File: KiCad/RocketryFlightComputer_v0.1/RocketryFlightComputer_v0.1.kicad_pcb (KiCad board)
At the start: 4 copper layers, 25.4 x 31.8 mm, 34 parts, among them J1 USB_C_Receptacle, J2 Conn_Coaxial, J3 DEPLOYMENT, J4 POWER_IN, Q1 BSS806NH6327XTSA1, Q2 BSS806NH6327XTSA1, Q3 BSS806NH6327XTSA1, U1 STM32U545RET6Q, U2 SX1262IMLTRT, U3 W25N01GWZEIG, U4 BME680, U5 MMC5633NJL, U6 TLV77118PDBVR, U7 ICM-20602, U8 TPS63070RNMR, U9 EVA-M8M-0, Y1 END4263D-32M, Y2 SIT1552AI-JE-DCC-32.768E

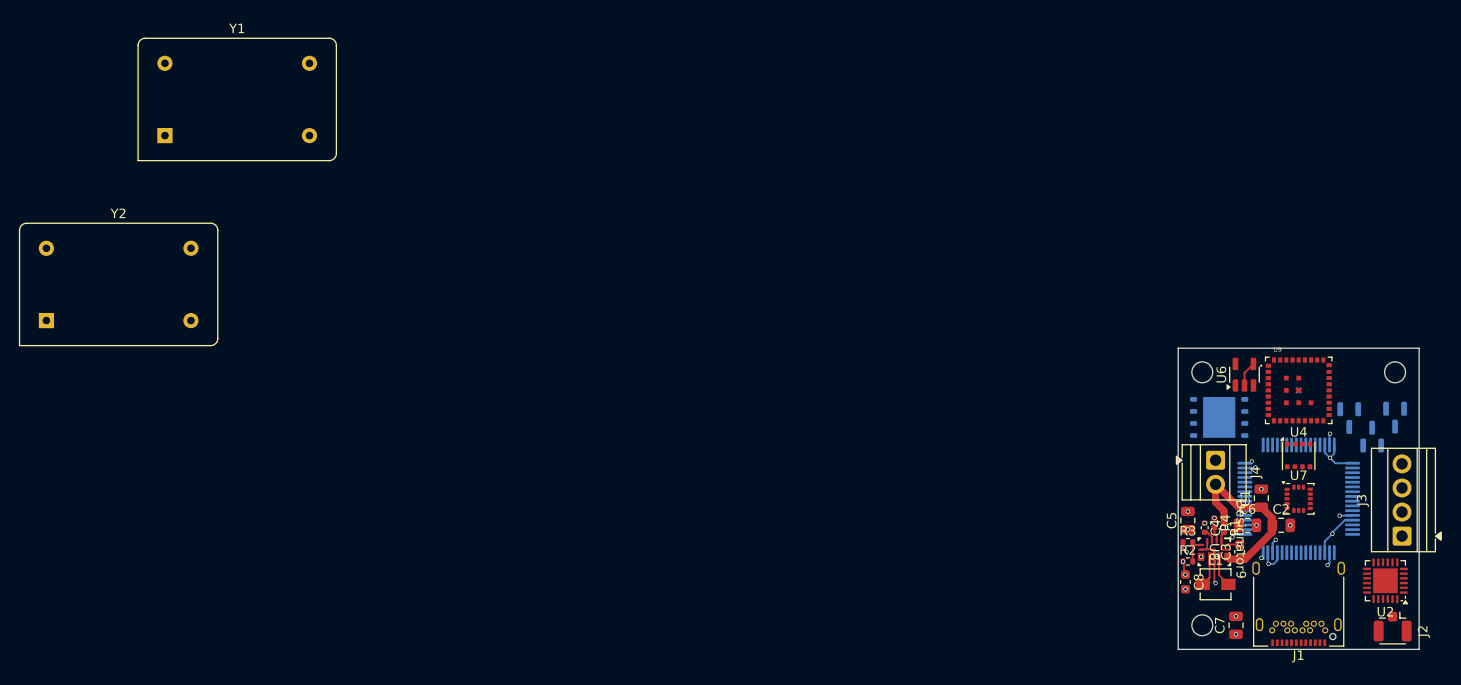
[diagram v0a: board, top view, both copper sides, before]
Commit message: Finished Board v0.1
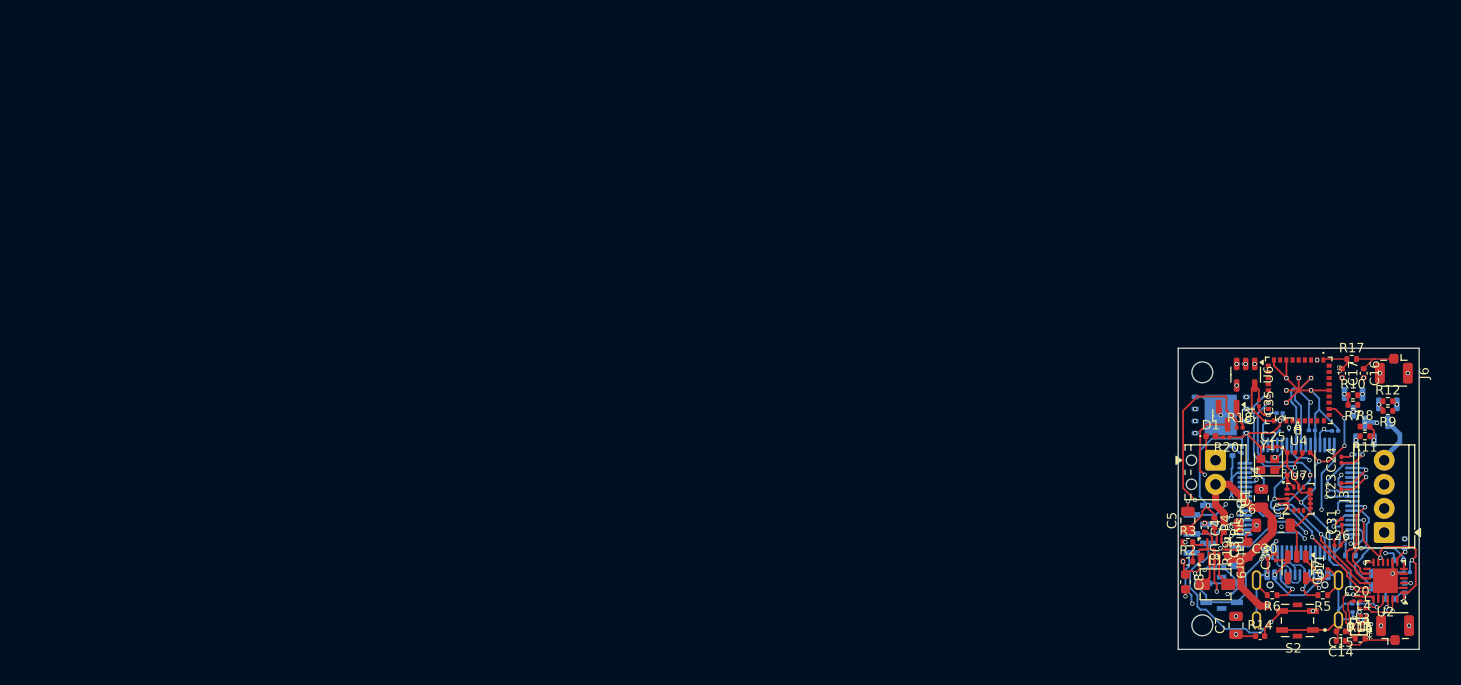
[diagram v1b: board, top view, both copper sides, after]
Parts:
- removed the REF** at (226.1, 88.3)
- added C10: 2.2u, Resistor_SMD:R_0402_1005Metric, B.Cu at (208.9, 96.5)
- added C11: 10p, Resistor_SMD:R_0402_1005Metric, B.Cu at (227.1, 111.0)
- added C12: 100n, Resistor_SMD:R_0402_1005Metric, B.Cu at (226.4, 108.1)
- added C13: 470u, Capacitor_SMD:C_0402_1005Metric, B.Cu at (227.1, 106.3)
- added C14: 0, Capacitor_SMD:C_0402_1005Metric, F.Cu at (220.3, 116.6)
- added C15: 0, Capacitor_SMD:C_0402_1005Metric, F.Cu at (220.3, 115.6)
- added C16: 0, Capacitor_SMD:C_0402_1005Metric, F.Cu at (222.8, 88.4)
- added C17: 0, Capacitor_SMD:C_0402_1005Metric, F.Cu at (220.5, 88.4)
- added C18: 1.5p, Capacitor_SMD:C_0201_0603Metric, B.Cu at (221.9, 113.5)
- added C19: 1p, Capacitor_SMD:C_0201_0603Metric, B.Cu at (222.4, 114.3)
- added C20: 1p, Capacitor_SMD:C_0201_0603Metric, F.Cu at (222.0, 112.4)
- added C21: 100p, Capacitor_SMD:C_0201_0603Metric, B.Cu at (224.4, 114.6)
- added C22: 100n, Capacitor_SMD:C_0201_0603Metric, B.Cu at (219.7, 94.4)
- added C23: 10u, Capacitor_SMD:C_0201_0603Metric, F.Cu at (220.4, 100.3)
- added C24: 10u, Capacitor_SMD:C_0201_0603Metric, F.Cu at (220.4, 97.5)
- added C25: 4.7u, Capacitor_SMD:C_0201_0603Metric, F.Cu at (213.2, 96.1)
- added C26: 1u, Capacitor_SMD:C_0201_0603Metric, F.Cu at (220.0, 106.5)
- added C27: 100n, Capacitor_SMD:C_0201_0603Metric, B.Cu at (222.1, 96.9)
- added C28: 100n, Capacitor_SMD:C_0201_0603Metric, B.Cu at (217.3, 94.4)
- added C29: 100n, Capacitor_SMD:C_0201_0603Metric, B.Cu at (209.9, 96.4)
- added C30: 100n, Capacitor_SMD:C_0201_0603Metric, F.Cu at (212.3, 107.9)
- added C31: 1u, Capacitor_SMD:C_0201_0603Metric, F.Cu at (220.4, 104.0)
- added C32: 2.2u, Capacitor_SMD:C_0201_0603Metric, B.Cu at (227.3, 109.3)
- added C33: 10u, Capacitor_SMD:C_0201_0603Metric, B.Cu at (213.9, 92.6)
- added C34: 10u, Capacitor_SMD:C_0201_0603Metric, B.Cu at (209.8, 87.4)
- added C35: 10u, Capacitor_SMD:C_0201_0603Metric, F.Cu at (211.7, 91.5)
- added C36: 2.2u, Capacitor_SMD:C_0201_0603Metric, F.Cu at (213.5, 107.8)
- added C37: 2.2u, Capacitor_SMD:C_0201_0603Metric, F.Cu at (218.9, 109.3)
- added C9: 2.2u, Resistor_SMD:R_0402_1005Metric, B.Cu at (221.4, 107.6)
- added D1: LED, LED_SMD:LED_0402_1005Metric, F.Cu at (206.6, 95.0)
- added J5: USB_C_Receptacle_USB2.0_16P, Connector_USB:USB_C_Receptacle_GCT_USB4105-xx-A_16P_TopMnt_Horizontal, B.Cu at (215.8, 113.3)
- added J6: Conn_Coaxial, Connector_Coaxial:U.FL_Hirose_U.FL-R-SMT-1_Vertical, F.Cu at (225.9, 87.9)
- added L2: 2.2u, Capacitor_SMD:C_0805_2012Metric, B.Cu at (209.4, 107.6)
- added L3: 3.9n, Inductor_SMD:L_0201_0603Metric, F.Cu at (222.6, 113.2)
- added L4: 6.8n, Inductor_SMD:L_0201_0603Metric, F.Cu at (222.8, 113.9)
- added L5: 8.2n, Inductor_SMD:L_0201_0603Metric, B.Cu at (221.9, 112.6)
- added Q4: BSS806NH6327XTSA1, Package_TO_SOT_SMD:SOT-23, F.Cu at (208.4, 92.8)
- added R10: 10k, Resistor_SMD:R_0402_1005Metric, F.Cu at (221.6, 90.7)
- added R11: 10k, Resistor_SMD:R_0402_1005Metric, F.Cu at (222.9, 95.0)
- added R12: 10k, Resistor_SMD:R_0402_1005Metric, F.Cu at (225.3, 91.3)
- added R13: 220, Resistor_SMD:R_0402_1005Metric, B.Cu at (225.6, 112.1)
- added R14: 10k, Capacitor_SMD:C_0402_1005Metric, F.Cu at (211.8, 116.1)
- added R15: 10k, Capacitor_SMD:C_0402_1005Metric, B.Cu at (207.5, 108.8)
- added R16: 0, Resistor_SMD:R_0402_1005Metric, F.Cu at (222.4, 116.3)
- added R17: 0, Resistor_SMD:R_0402_1005Metric, F.Cu at (221.5, 86.9)
- added R18: 10k, Resistor_SMD:R_0201_0603Metric, F.Cu at (209.7, 94.1)
- added R19: 100k, Resistor_SMD:R_0201_0603Metric, F.Cu at (209.4, 107.3)
- added R20: 330, Resistor_SMD:R_0201_0603Metric, F.Cu at (208.3, 95.1)
- added R5: 5.1k, Resistor_SMD:R_0402_1005Metric, F.Cu at (218.4, 111.8)
- added R6: 5.1k, Resistor_SMD:R_0402_1005Metric, F.Cu at (213.1, 111.8)
- added R7: 100, Resistor_SMD:R_0402_1005Metric, F.Cu at (221.6, 91.7)
- added R8: 100, Resistor_SMD:R_0402_1005Metric, F.Cu at (222.9, 94.0)
- added R9: 100, Resistor_SMD:R_0402_1005Metric, F.Cu at (225.3, 92.3)
- added S1: TS21-34-035-BK-160-SMT-TR, Footprints:SW_TS21-34-035-BK-160-SMT-TR, B.Cu at (207.8, 111.5)
- added S2: TS21-34-035-BK-160-SMT-TR, Footprints:SW_TS21-34-035-BK-160-SMT-TR, F.Cu at (215.8, 114.4)
- added U10: SKY13453-385LF, Footprints:QFN_453-385LF_SKY, F.Cu at (222.2, 115.1)
- added U11: TLV75733PDBV, Package_TO_SOT_SMD:SOT-23-5, F.Cu at (215.7, 108.8)
- added XTAL1: SIT1552AI-JE-DCC-32.768E, Footprints:BGA4_SiT1532_SIT, B.Cu at (214.4, 94.2)
- J1: value USB_C_Receptacle -> Conn_01x06_Pin; footprint Connector_USB:USB_C_Receptacle_Amphenol_12401548E4-2A -> Connector_PinHeader_1.00mm:PinHeader_1x06_P1.00mm_Vertical_SMD_Pin1Left; moved to B.Cu
- J3: footprint TerminalBlock:TerminalBlock_Xinya_XY308-2.54-4P_1x04_P2.54mm_Horizontal -> TerminalBlock_Phoenix:TerminalBlock_Phoenix_MPT-0,5-4-2.54_1x04_P2.54mm_Horizontal
- J4: footprint TerminalBlock:TerminalBlock_Xinya_XY308-2.54-2P_1x02_P2.54mm_Horizontal -> TerminalBlock_Phoenix:TerminalBlock_Phoenix_MPT-0,5-2-2.54_1x02_P2.54mm_Horizontal
- Y1: value END4263D-32M -> ECS-2520MV-xxx-xx; footprint Oscillator:Oscillator_DIP-14 -> Crystal:Crystal_SMD_SeikoEpson_FA128-4Pin_2.0x1.6mm
- Y2: value SIT1552AI-JE-DCC-32.768E -> TG2520SMN; footprint Oscillator:Oscillator_DIP-14 -> Oscillator:Oscillator_SMD_SeikoEpson_TG2520SMN-xxx-xxxxxx-4Pin_2.5x2.0mm; moved to B.Cu
- moved Y2 143.5 mm to (224.8, 110.2), turned to -90 degrees
- moved Y1 121.3 mm to (212.6, 98.0)
- moved J1 12.5 mm to (205.5, 104.8)
- moved J3 1.91 mm to (224.9, 105.2)
- moved Q1 1.66 mm to (221.7, 91.5)
- moved Q2 0.94 mm to (222.9, 94.5)
- moved C3 0.92 mm to (210.6, 106.9)
- moved Q3 0.89 mm to (225.3, 92.6)
- moved U4 0.89 mm to (215.9, 97.9)
- moved J2 0.46 mm to (226.1, 115.4), turned to 90 degrees
- moved U3 0.30 mm to (207.7, 92.8)
- moved U6 0.13 mm to (210.3, 88.5), turned to -90 degrees
- turned U1 to -90 degrees
- turned U9 to -90 degrees
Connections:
- C1 pad 1: Net-(J4-Pin_2) -> +BATT
- C2 pad 1: Net-(J4-Pin_2) -> +BATT
- C3 pad 1: Net-(J4-Pin_2) -> +BATT
- J3 pad 1: unconnected-(J3-Pin_1-Pad1) -> +BATT
- J3 pad 2: unconnected-(J3-Pin_2-Pad2) -> Net-(J3-Pin_2)
- J3 pad 3: unconnected-(J3-Pin_3-Pad3) -> Net-(J3-Pin_3)
- J3 pad 4: unconnected-(J3-Pin_4-Pad4) -> Net-(J3-Pin_4)
- J4 pad 2: Net-(J4-Pin_2) -> +BATT
- Q1 pad 1: unconnected-(Q1-G-Pad1) -> Net-(Q1-G)
- Q1 pad 2: unconnected-(Q1-S-Pad2) -> GND
- Q1 pad 3: unconnected-(Q1-D-Pad3) -> Net-(J3-Pin_2)
- Q2 pad 1: unconnected-(Q2-G-Pad1) -> Net-(Q2-G)
- Q2 pad 2: unconnected-(Q2-S-Pad2) -> GND
- Q2 pad 3: unconnected-(Q2-D-Pad3) -> Net-(J3-Pin_3)
- Q3 pad 1: unconnected-(Q3-G-Pad1) -> Net-(Q3-G)
- Q3 pad 2: unconnected-(Q3-S-Pad2) -> GND
- Q3 pad 3: unconnected-(Q3-D-Pad3) -> Net-(J3-Pin_4)
- R1 pad 1: Net-(J4-Pin_2) -> +BATT
- R1 pad 2: Net-(U8-EN) -> Net-(U8-PS_SYNC)
- U1 pad 16: unconnected-(U1-PA2-Pad16) -> QSPI_CSN
- U1 pad 17: unconnected-(U1-PA3-Pad17) -> QSPI_CLK
- U1 pad 22: unconnected-(U1-PA6-Pad22) -> QSPI_D3
- U1 pad 23: unconnected-(U1-PA7-Pad23) -> QSPI_D2
- U1 pad 24: unconnected-(U1-PB0-Pad24) -> QSPI_D1
- U1 pad 25: unconnected-(U1-PB1-Pad25) -> QSPI_D0
- U1 pad 26: unconnected-(U1-PB2-Pad26) -> SX_NRST
- U1 pad 27: unconnected-(U1-PB10-Pad27) -> SX_BUSY
- U1 pad 28: unconnected-(U1-VLXSMPS-Pad28) -> V_SMPS
- U1 pad 3: unconnected-(U1-PC14-Pad3) -> Net-(U1-PC14)
- U1 pad 31: VDD -> Net-(C10-Pad1)
- U1 pad 34: unconnected-(U1-PB13-Pad34) -> SCK
- U1 pad 35: unconnected-(U1-PB14-Pad35) -> MISO
- U1 pad 36: unconnected-(U1-PB15-Pad36) -> MOSI
- U1 pad 37: unconnected-(U1-PC6-Pad37) -> SX_CSN
- U1 pad 44: unconnected-(U1-PA11-Pad44) -> USB_D-
- U1 pad 45: unconnected-(U1-PA12-Pad45) -> USB_D+
- U1 pad 46: unconnected-(U1-PA13-Pad46) -> SWDIO
- U1 pad 49: unconnected-(U1-PA14-Pad49) -> SWCLK
- U1 pad 5: unconnected-(U1-PH0-Pad5) -> Net-(U1-PH0)
- U1 pad 55: unconnected-(U1-PB3-Pad55) -> SWO
- U1 pad 60: unconnected-(U1-PH3-Pad60) -> BOOT0
- U1 pad 62: VDD -> Net-(C10-Pad1)
- U1 pad 7: unconnected-(U1-NRST-Pad7) -> NRST
- U1 pad 8: unconnected-(U1-PC0-Pad8) -> SCL
- U1 pad 9: unconnected-(U1-PC1-Pad9) -> SDA
- U2 pad 1: unconnected-(U2-VDD_IN-Pad1) -> VDD
- U2 pad 10: unconnected-(U2-VBAT-Pad10) -> VDD
- U2 pad 11: unconnected-(U2-VBAT_IO-Pad11) -> VDD
- U2 pad 12: unconnected-(U2-DIO2-Pad12) -> RF_SW_CTRL
- U2 pad 13: unconnected-(U2-DIO1-Pad13) -> SX_IRQ
- U2 pad 14: unconnected-(U2-BUSY-Pad14) -> SX_BUSY
- U2 pad 15: unconnected-(U2-~{RESET}-Pad15) -> SX_NRST
- U2 pad 16: unconnected-(U2-MISO-Pad16) -> MISO
- U2 pad 17: unconnected-(U2-MOSI-Pad17) -> MOSI
- U2 pad 18: unconnected-(U2-SCK-Pad18) -> SCK
- U2 pad 19: unconnected-(U2-NSS-Pad19) -> SX_CSN
- U2 pad 2: Net-(U2-GND-Pad2) -> GND
- U2 pad 20: Net-(U2-GND-Pad2) -> GND
- U2 pad 21: unconnected-(U2-RFI_P-Pad21) -> RFI_P
- U2 pad 22: unconnected-(U2-RFI_N-Pad22) -> RFI_N
- U2 pad 23: Net-(J2-In) -> RF_O
- U2 pad 24: unconnected-(U2-VR_PA-Pad24) -> VR_PA
- U2 pad 25: Net-(U2-GND-Pad2) -> GND
- U2 pad 3: unconnected-(U2-XTA-Pad3) -> Net-(U2-XTA)
- U2 pad 5: Net-(U2-GND-Pad2) -> GND
- U2 pad 6: unconnected-(U2-DIO3-Pad6) -> Net-(U2-DIO3)
- U2 pad 7: unconnected-(U2-VREG-Pad7) -> Net-(U2-VREG)
- U2 pad 8: Net-(U2-GND-Pad2) -> GND
- U3 pad 1: unconnected-(U3-~{CS}-Pad1) -> QSPI_CSN
- U3 pad 2: unconnected-(U3-DO/IO_{1}-Pad2) -> QSPI_D1
- U3 pad 3: unconnected-(U3-~{WP}/IO_{2}-Pad3) -> QSPI_D2
- U3 pad 4: unconnected-(U3-GND-Pad4) -> GND
- U3 pad 5: unconnected-(U3-DI/IO_{0}-Pad5) -> QSPI_D0
- U3 pad 6: unconnected-(U3-CLK-Pad6) -> QSPI_CLK
- U3 pad 7: unconnected-(U3-~{HOLD}/~{RESET}/IO_{3}-Pad7) -> QSPI_D3
- U3 pad 8: unconnected-(U3-VCC-Pad8) -> VDD
- U3 pad 9: unconnected-(U3-EP-Pad9) -> GND
- U4 pad 1: unconnected-(U4-GND-Pad1) -> GND
- U4 pad 2: unconnected-(U4-CSB-Pad2) -> BME_CSN
- U4 pad 3: unconnected-(U4-SDI-Pad3) -> MOSI
- U4 pad 4: unconnected-(U4-SCK-Pad4) -> SCK
- U4 pad 5: unconnected-(U4-SDO-Pad5) -> MISO
- U4 pad 6: unconnected-(U4-VDDIO-Pad6) -> VDD
- U4 pad 7: unconnected-(U4-GND-Pad7) -> GND
- U4 pad 8: unconnected-(U4-VDD-Pad8) -> VDD
- U5 pad A1: unconnected-(U5-VSA-PadA1) -> GND
- U5 pad A2: unconnected-(U5-SCL-PadA2) -> SCL
- U5 pad B1: unconnected-(U5-VDD-PadB1) -> VDD
- U5 pad B2: unconnected-(U5-SDA-PadB2) -> SDA
- U6 pad 1: unconnected-(U6-IN-Pad1) -> VDD
- U6 pad 2: Net-(U6-GND-Pad2) -> GND
- U6 pad 3: unconnected-(U6-EN-Pad3) -> VDD
- U6 pad 4: Net-(U6-GND-Pad2) -> GND
- U6 pad 5: unconnected-(U6-OUT-Pad5) -> +1V8
- U7 pad 1: unconnected-(U7-VDDIO-Pad1) -> VDD
- U7 pad 10: Net-(U7-GND-Pad10) -> GND
- U7 pad 11: Net-(U7-GND-Pad10) -> GND
- U7 pad 12: Net-(U7-GND-Pad10) -> GND
- U7 pad 13: Net-(U7-GND-Pad10) -> GND
- U7 pad 15: Net-(U7-GND-Pad10) -> GND
- U7 pad 16: unconnected-(U7-VDD-Pad16) -> VDD
- U7 pad 2: unconnected-(U7-SCL/SPC-Pad2) -> SCK
- U7 pad 3: unconnected-(U7-SDA/SDI-Pad3) -> MOSI
- U7 pad 4: unconnected-(U7-SAO/SD0-Pad4) -> MISO
- U7 pad 5: unconnected-(U7-~{CS}-Pad5) -> ICM_CSN
- U7 pad 9: Net-(U7-GND-Pad10) -> GND
- U8 pad 1: Net-(U8-EN) -> Net-(U8-PS_SYNC)
- U8 pad 12: Net-(J4-Pin_2) -> +BATT
- U8 pad 13: Net-(J4-Pin_2) -> +BATT
- U8 pad 14: Net-(U8-EN) -> 3V3_EN
- U9 pad 1: unconnected-(U9-RF_IN-Pad1) -> Net-(U9-RF_IN)
- U9 pad 15: unconnected-(U9-RXD/SPI_MOSI-Pad15) -> MOSI
- U9 pad 16: unconnected-(U9-TXD/SPI_MISO-Pad16) -> MISO
- U9 pad 18: unconnected-(U9-GND__1-Pad18) -> GND
- U9 pad 19: unconnected-(U9-VCC-Pad19) -> +1V8
- U9 pad 2: unconnected-(U9-GND-Pad2) -> GND
- U9 pad 20: unconnected-(U9-VCC_IO-Pad20) -> VDD
- U9 pad 29: unconnected-(U9-SCL/SPI_CLK-Pad29) -> SCK
- U9 pad 30: unconnected-(U9-SDA/SPI_CS_N-Pad30) -> GPS_CSN
- U9 pad 32: unconnected-(U9-D_SEL-Pad32) -> GND
- U9 pad 37: unconnected-(U9-GND__2-Pad37) -> GND
- U9 pad 38: unconnected-(U9-GND__3-Pad38) -> GND
- U9 pad 39: unconnected-(U9-GND__4-Pad39) -> GND
- U9 pad 40: unconnected-(U9-GND__5-Pad40) -> GND
- U9 pad 41: unconnected-(U9-GND__6-Pad41) -> GND
- U9 pad 42: unconnected-(U9-GND__7-Pad42) -> GND
- U9 pad 43: unconnected-(U9-GND__8-Pad43) -> GND
- U9 pad 7: unconnected-(U9-VDD_USB-Pad7) -> GND
- U9 pad 9: unconnected-(U9-RTC_I-Pad9) -> GND
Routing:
- net VDD: track 18.4 -> 161.3 mm, vias 11 -> 23
- net GND: track 15.0 -> 141.1 mm, vias 16 -> 40
- net +BATT: track 0.00 -> 55.7 mm, vias 0 -> 1
- net NRST: track 0.00 -> 50.4 mm, vias 0 -> 4
- net USB_VBUS: track 0.00 -> 46.4 mm, vias 0 -> 3
- net MOSI: track 0.00 -> 36.8 mm, vias 0 -> 4
- net BOOT0: track 0.00 -> 35.5 mm, vias 0 -> 2
- net Net-(C10-Pad1): track 0.00 -> 34.5 mm, vias 0 -> 4
- net MISO: track 0.00 -> 34.3 mm, vias 0 -> 4
- net SCK: track 0.00 -> 30.1 mm, vias 0 -> 5
- net SWO: track 0.00 -> 28.6 mm, vias 0 -> 2
- net QSPI_CSN: track 0.00 -> 24.0 mm, vias 0 -> 2
- net QSPI_D0: track 0.00 -> 23.1 mm, vias 0 -> 2
- net QSPI_D2: track 0.00 -> 20.2 mm, vias 0 -> 2
- net QSPI_D1: track 0.00 -> 19.9 mm, vias 0 -> 2
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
